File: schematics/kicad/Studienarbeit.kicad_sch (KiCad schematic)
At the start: 43 parts, among them J1 Barrel_Jack_Switch, U1 ESP32-WROOM-32E, U2 PCM5102, U3 MCP6001-OT, U4 MCP6001-OT, U5 MCP6001, U6 TPA711

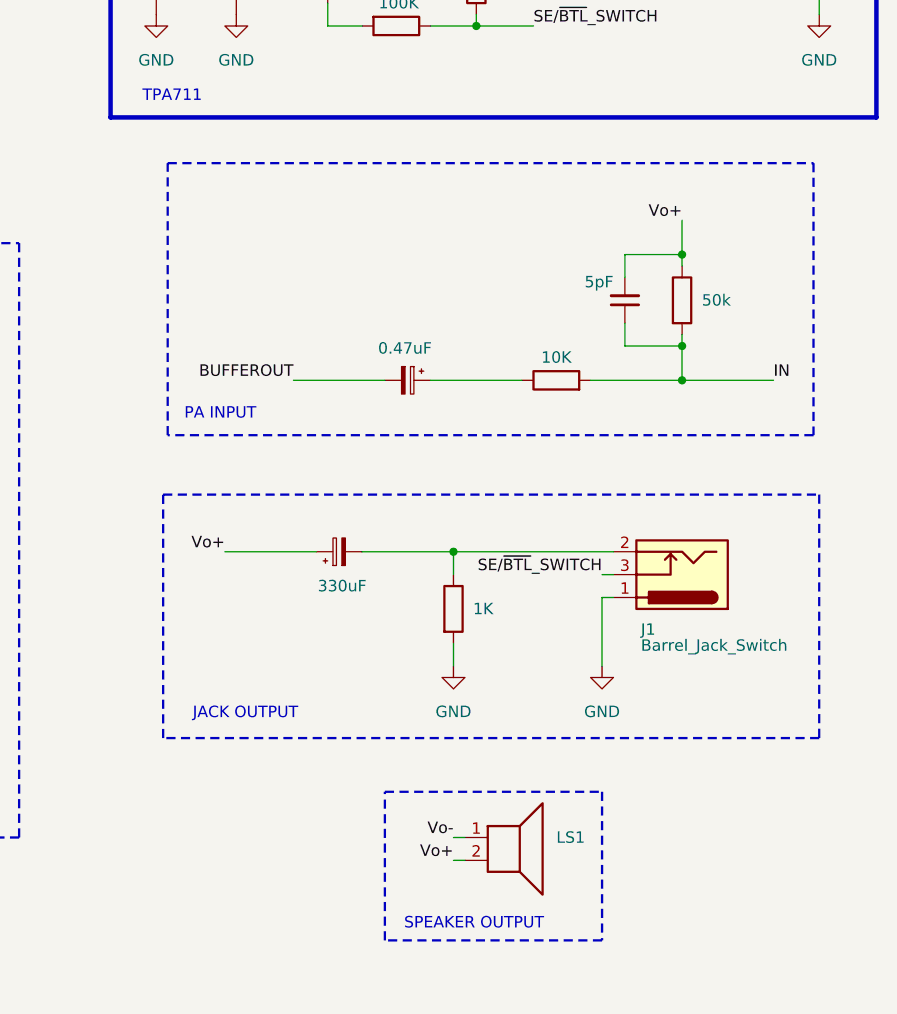
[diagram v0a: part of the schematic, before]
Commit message: Added ESP32 Footprint.
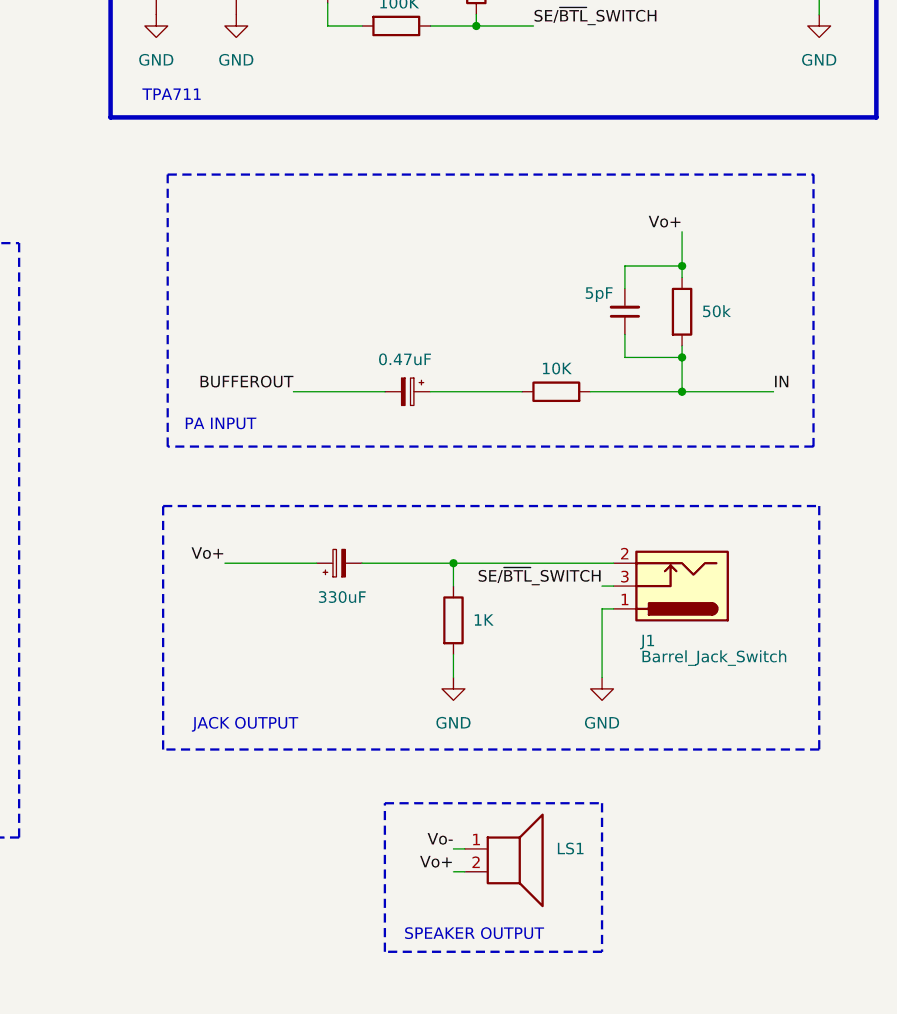
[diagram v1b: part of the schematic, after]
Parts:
- U3, U4: footprint MCP6001_SOT23-5:SOT23-5 -> Package_TO_SOT_SMD:SOT-23-5
- U5: footprint MCP6001:SOT23-5 -> Package_TO_SOT_SMD:SOT-23-5
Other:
- moved on the sheet: J1, LS1

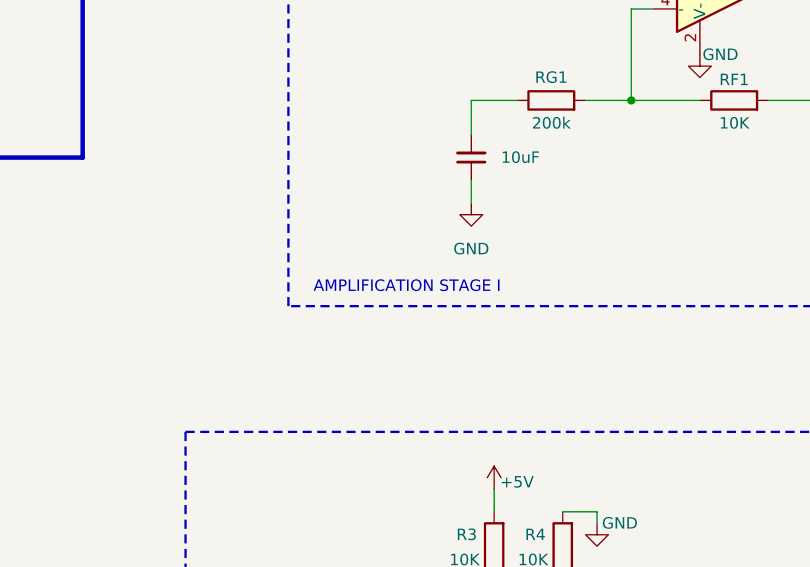
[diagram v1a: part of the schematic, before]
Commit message: KiCad: Draft of PCB.
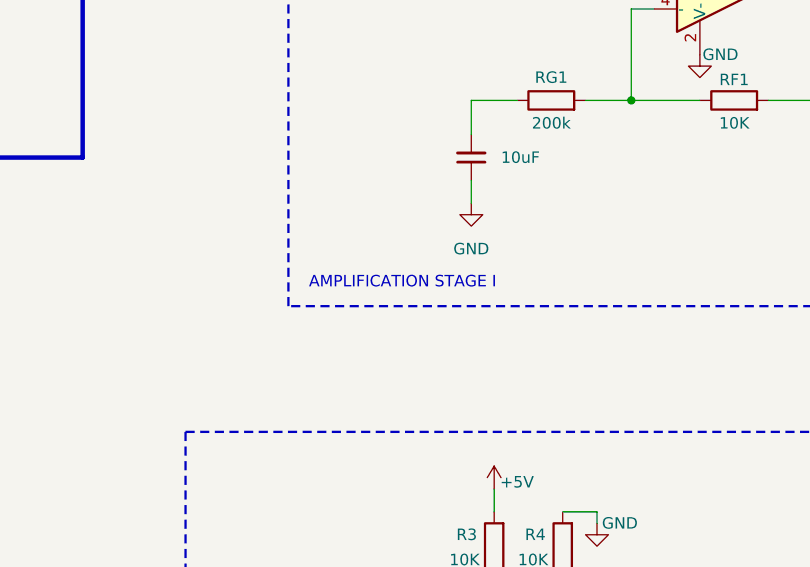
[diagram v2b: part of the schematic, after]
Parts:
- U1: footprint RF_Module:ESP32-WROOM-32D -> RF_Module:ESP32-WROOM-32E
- U6: footprint Package_DFN_QFN:Texas_DRB0008A -> Package_SO:Texas_DGN0008D_VSSOP-8-1EP_3x3mm_P0.65mm_EP2x2.94mm_Mask1.57x1.89mm
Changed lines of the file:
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@@
 	(text "AMPLIFICATION STAGE I"
 		(exclude_from_sim no)
-		(at 208.788 142.748 0)
+		(at 208.28 142.24 0)
 		(effects
 			(font
@@
 			)
 		)
-		(property "Footprint" "RF_Module:ESP32-WROOM-32D"
+		(property "Footprint" "RF_Module:ESP32-WROOM-32E"
 			(at 57.15 200.66 0)
 			(effects
@@
 			)
 		)
-		(property "Footprint" "Package_DFN_QFN:Texas_DRB0008A"
+		(property "Footprint" "Package_SO:Texas_DGN0008D_VSSOP-8-1EP_3x3mm_P0.65mm_EP2x2.94mm_Mask1.57x1.89mm"
 			(at 373.38 121.92 0)
 			(effects
